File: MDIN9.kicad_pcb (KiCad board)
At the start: 2 copper layers, 110 x 50 mm, 40 parts, among them CN1 9, CN2 9, CN3 35RAPC4BH3, CN5 B6B-XH-A(LF)(SN), CN6 353180620, J1A JAMMA PINS 3.96MM PITCH 2.2MM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, J1B JAMMA PINS 3.96MM PITCH 2.2MM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, SW1 MJTP1230, SW2 MJTP1230, SW3 A6H-4101, SW4 CL-SA-12C-02, U1 THS7374

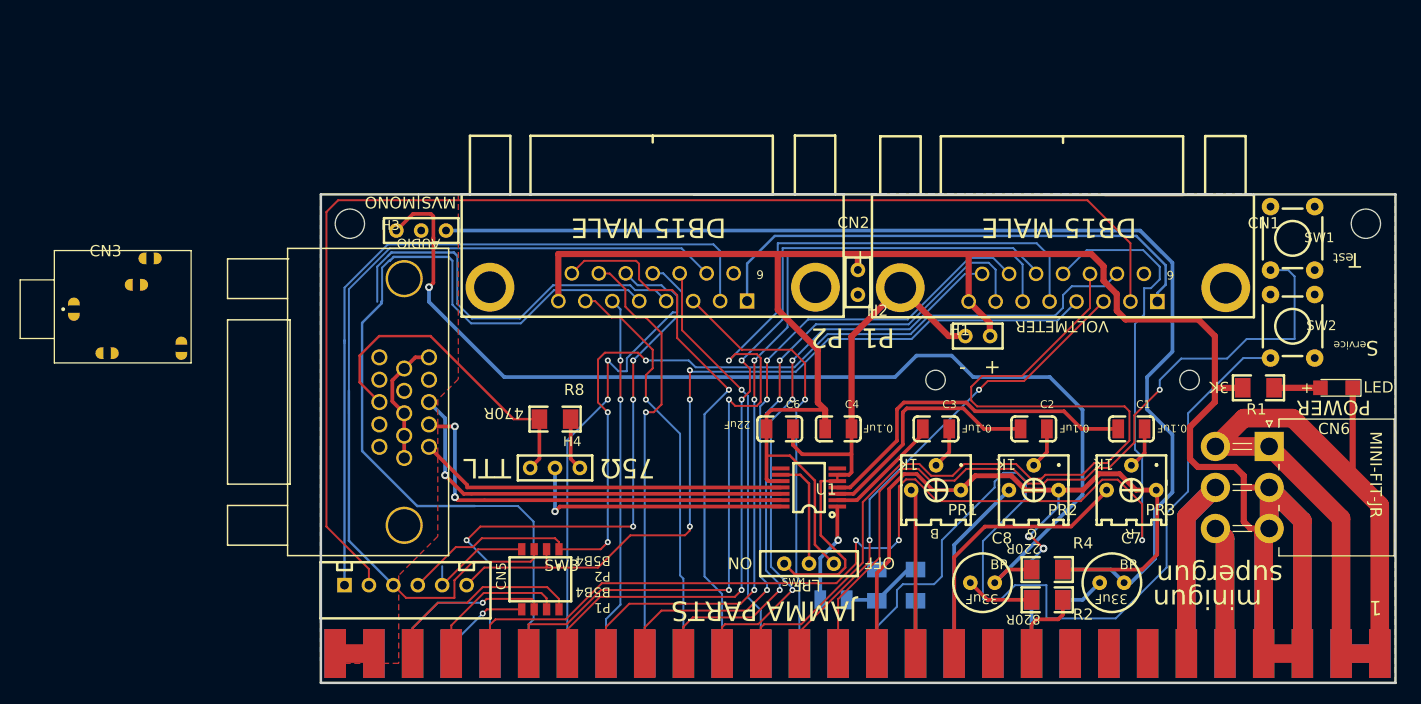
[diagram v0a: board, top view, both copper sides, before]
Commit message: Full route
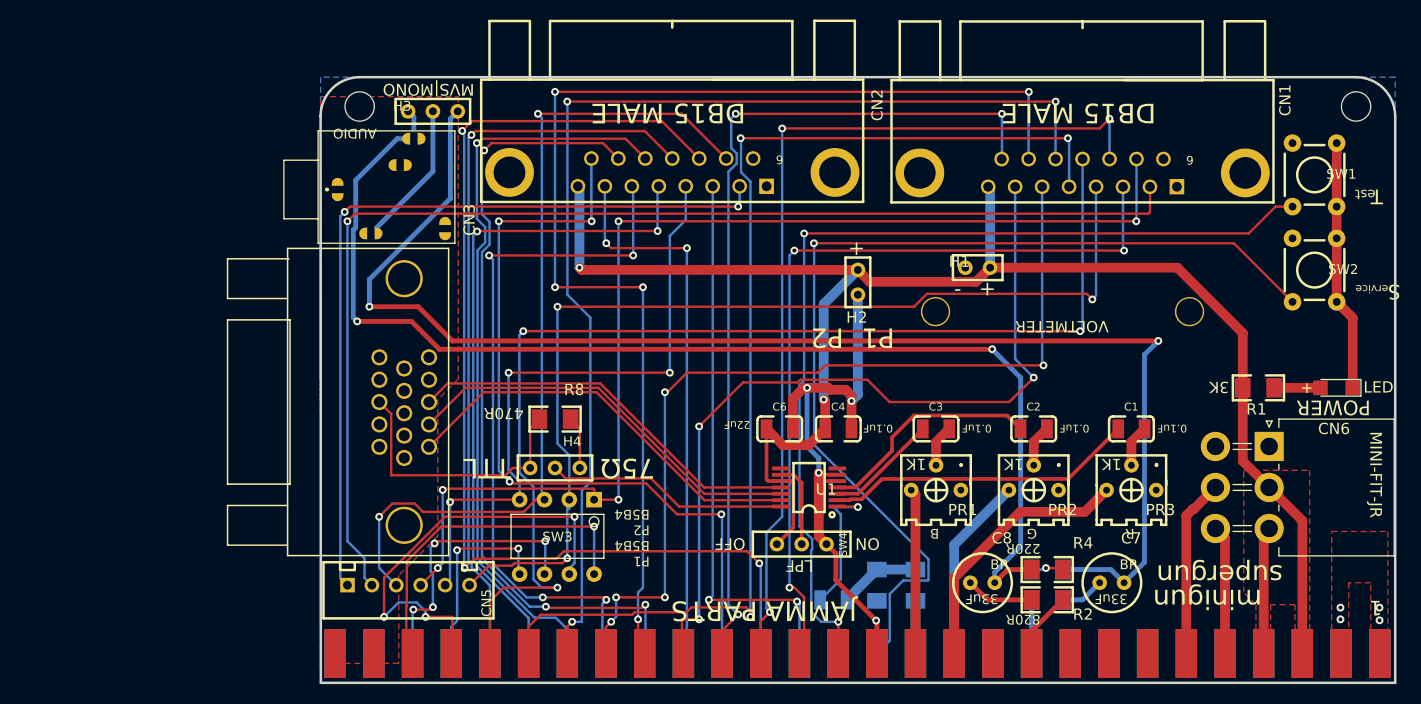
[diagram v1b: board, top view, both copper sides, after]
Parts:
- removed the ? at (3.00, -7.00)
- removed the ? at (107.0, -7.00)
- added ?: , AutoGenerated:MountingHole_3.00mm, F.Cu at (4.00, -19.0)
- added ?: , AutoGenerated:MountingHole_3.00mm, F.Cu at (106.0, -19.0)
- SW3: value A6H-4101 -> DIPSwitch-4; footprint easyeda:A6H-4101 -> MinigunParts:DIPSwitch-4
- moved CN3 29.6 mm to (6.75, -10.8)
- moved H3 12.3 mm to (11.5, -18.5)
- moved CN1 11.9 mm to (78.0, -12.2)
- moved CN2 11.9 mm to (36.0, -12.2)
- moved SW3 9.83 mm to (28.0, 21.2), turned to 270 degrees
- moved H1 7.00 mm to (67.3, -2.50)
- moved VOLTMETER 7.00 mm to (76.0, 2.00)
- moved SW1 6.88 mm to (101.8, -12.0)
- moved SW2 6.17 mm to (101.8, -2.25)
- moved SW4 2.14 mm to (49.2, 25.8), turned to 180 degrees
- moved CN5 0.30 mm to (9.00, 30.0)
- turned R7 to 270 degrees
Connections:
- SW3 pad 2: P1_B5_J -> P1_B4
- SW3 pad 3: P1_B4 -> P2_B5
- SW3 pad 4: P1_B4_J -> P2_B4
- SW3 pad 5: P2_B5 -> P2_B4_J
- SW3 pad 7: P2_B4 -> P1_B4_J
- SW3 pad 8: P2_B4_J -> P1_B5_J
- U1 pad 11: VIDEO_RED_3 -> VIDEO_GREEN_3
- U1 pad 12: VIDEO_GREEN_3 -> VIDEO_BLUE_3
- U1 pad 13: VIDEO_BLUE_3 -> VIDEO_RED_3
- U1 pad 2: VIDEO_BLUE_2 -> VIDEO_RED_2
- U1 pad 3: VIDEO_GREEN_2 -> VIDEO_BLUE_2
- U1 pad 4: VIDEO_RED_2 -> VIDEO_GREEN_2
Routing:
- net GND: track 293.1 -> 87.6 mm, vias 2 -> 9
- net P2_START: track 42.4 -> 111.8 mm, vias 1 -> 3
- net +5V: track 246.1 -> 177.5 mm, vias 0 -> 2
- net P1_LEFT: track 70.7 -> 122.4 mm, vias 3 -> 5
- net P2_LEFT: track 44.0 -> 81.2 mm, vias 1 -> 3
- net P2_RIGHT: track 37.0 -> 72.6 mm, vias 2 -> 4
- net P1_COIN: track 51.1 -> 82.9 mm, vias 2 -> 3
- net P1_UP: track 59.9 -> 89.0 mm
- net P1_B1: track 86.6 -> 114.9 mm
- net P1_B4_J: track 16.9 -> 44.9 mm, vias 0 -> 3
- net P2_UP: track 54.4 -> 80.4 mm, vias 1 -> 4
- net P2_B1: track 50.4 -> 76.3 mm, vias 2 -> 1
- net P1_B4: track 86.1 -> 105.7 mm
- net P2_B2: track 88.0 -> 68.8 mm, vias 0 -> 2
- net SP-_3: track 119.9 -> 139.0 mm, vias 0 -> 2
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- added copper zone on F.Cu, net +5V
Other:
- board size 110 x 50 mm -> 110 x 62 mm
- board text added: "ADVANCED EDITION + HD15 RGBS"
- board text added: "CS"
- board text removed: "ADVANCED EDITION"
